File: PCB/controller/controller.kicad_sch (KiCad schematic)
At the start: 14 parts, among them U1 Raspberry_Pi_Pico, X1 Switch, Y1 Switch

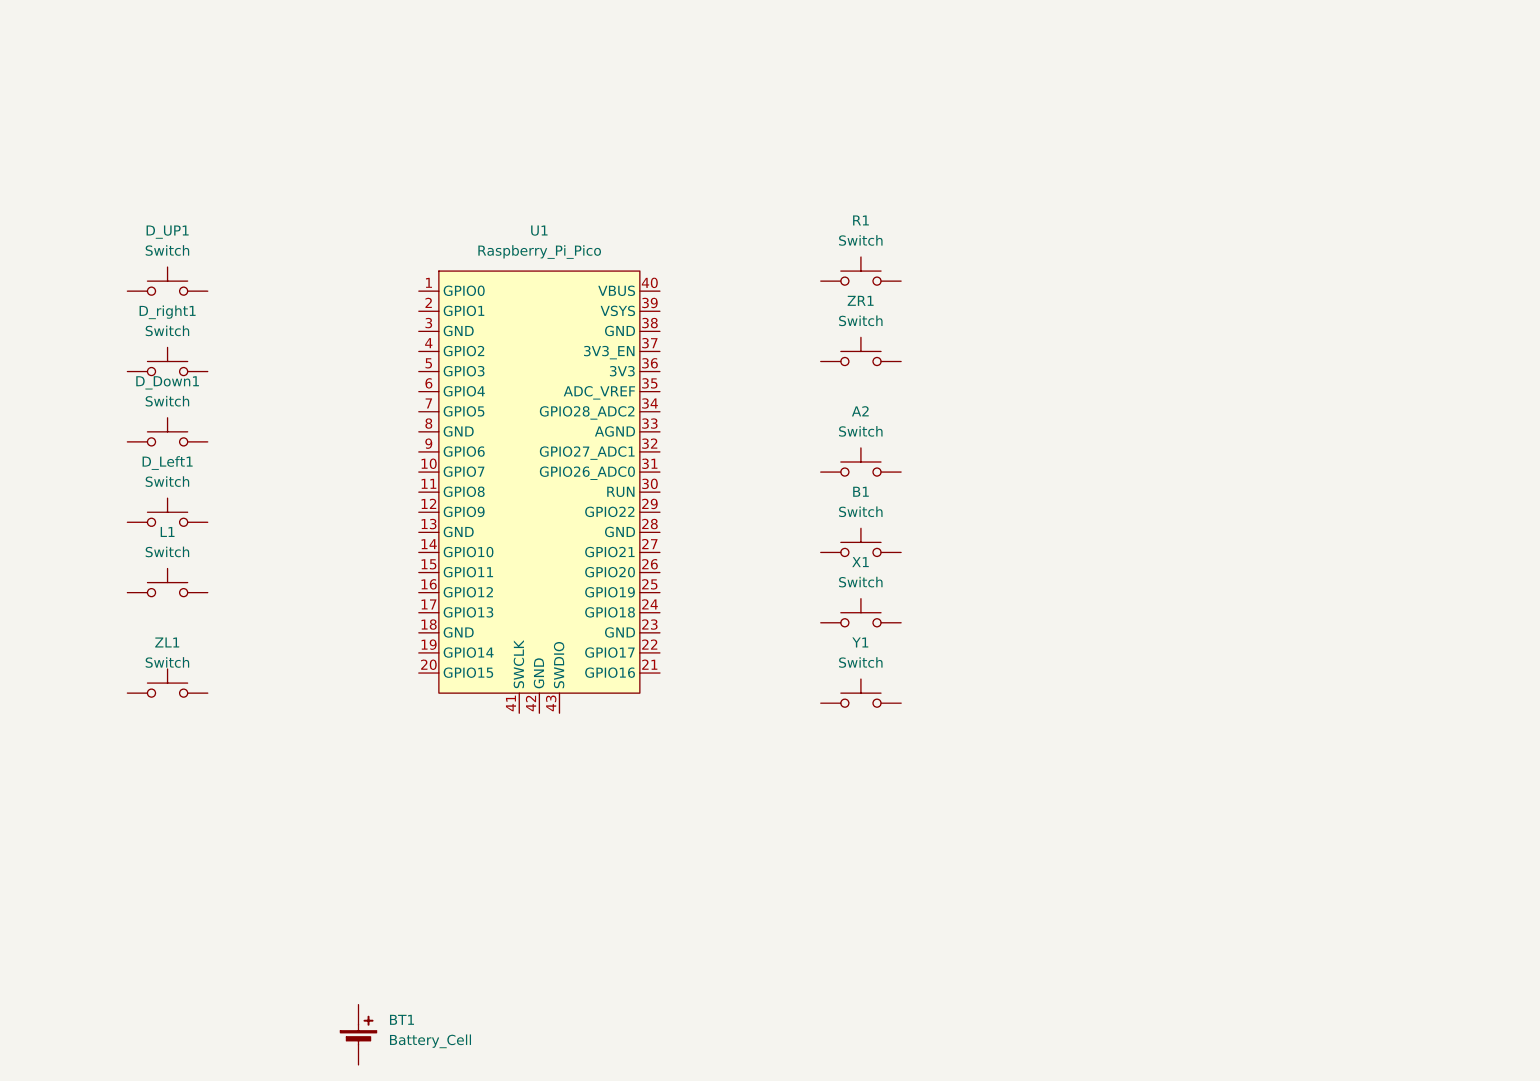
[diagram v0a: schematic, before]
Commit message: doin stuffs
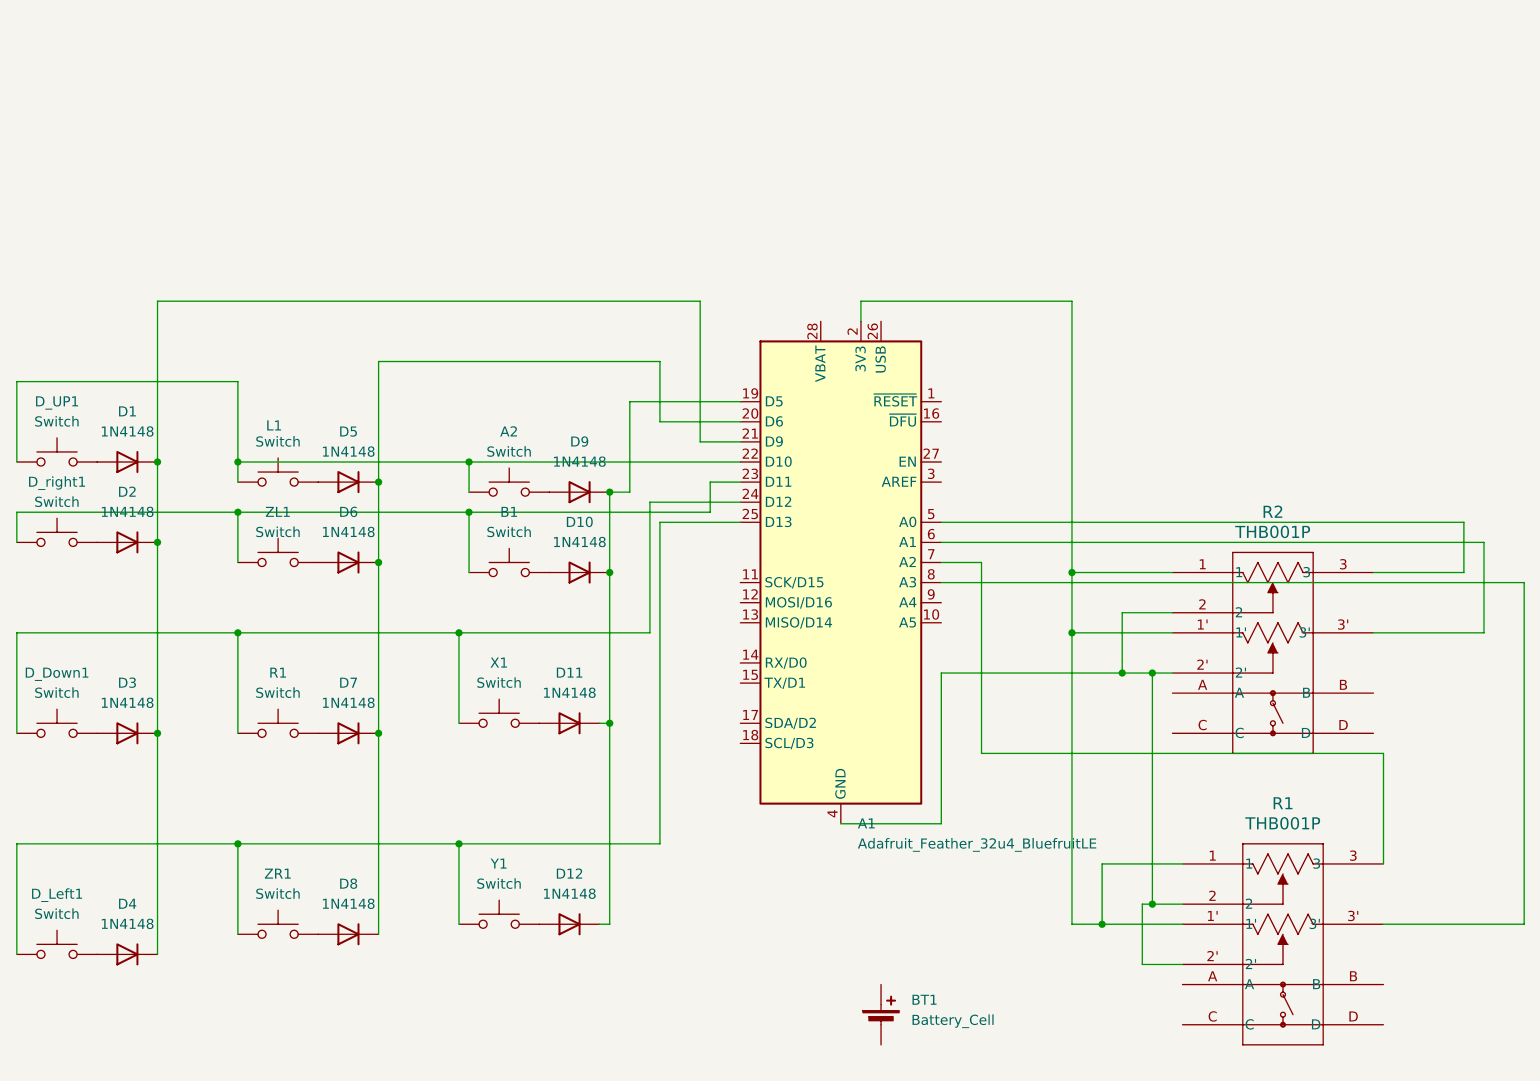
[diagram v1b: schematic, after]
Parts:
- removed U1: Raspberry_Pi_Pico, ScottoKeebs_MCU:Raspberry_Pi_Pico, symbol ScottoKeebs:MCU_Raspberry_Pi_Pico
- added A1: Adafruit_Feather_32u4_BluefruitLE, Module:Adafruit_Feather, symbol MCU_Module:Adafruit_Feather_32u4_BluefruitLE
- added D1, D10, D11, D12, D2, D3, D4, D5, D6, D7, D8, D9: 1N4148, Diode_THT:D_DO-35_SOD27_P7.62mm_Horizontal, symbol Diode:1N4148
- added R1, R2: THB001P, ScottoKeebs_Miscellaneous:THB001P_CNK, symbol 2025-05-29_23-49-57:THB001P
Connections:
- net at B1.1: now also D_right1.1, ZL1.1, A1.23 (D11)
- net at B1.2: now also D10.2 (A)
- net at A2.1: now also D_UP1.1, L1.1, A1.22 (D10)
- net at A2.2: now also D9.2 (A)
- net at ZR1.1: now also D_Left1.1, Y1.1, A1.25 (D13)
- net at ZR1.2: now also D8.2 (A)
- net at R1.1: now also D_Down1.1, X1.1, A1.24 (D12)
- net at R1.2: now also D7.2 (A)
- net at Y1.2: now also D12.2 (A)
- net at D_Down1.2: now also D3.2 (A)
- net at ZL1.2: now also D6.2 (A)
- net at D_right1.2: now also D2.2 (A)
- net at D_Left1.2: now also D4.2 (A)
- net at D_UP1.2: now also D1.2 (A)
- net at X1.2: now also D11.2 (A)
- net at L1.2: now also D5.2 (A)
- new net: A1.19 (D5), D10.1 (K), D11.1 (K), D12.1 (K), D9.1 (K)
- new net: A1.2 (3V3), R1.1, R1.1', R2.1, R2.1'
- new net: A1.20 (D6), D5.1 (K), D6.1 (K), D7.1 (K), D8.1 (K)
- new net: A1.21 (D9), D1.1 (K), D2.1 (K), D3.1 (K), D4.1 (K)
- new net: A1.4 (GND), R1.2, R1.2', R2.2, R2.2'
- new net: A1.5 (A0), R2.3
- new net: A1.6 (A1), R2.3'
- new net: A1.7 (A2), R1.3
- new net: A1.8 (A3), R1.3'
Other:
- moved on the sheet: A2, B1, BT1, D_Down1, D_Left1, D_UP1, D_right1, L1, R1, X1, Y1, ZL1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

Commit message: more work
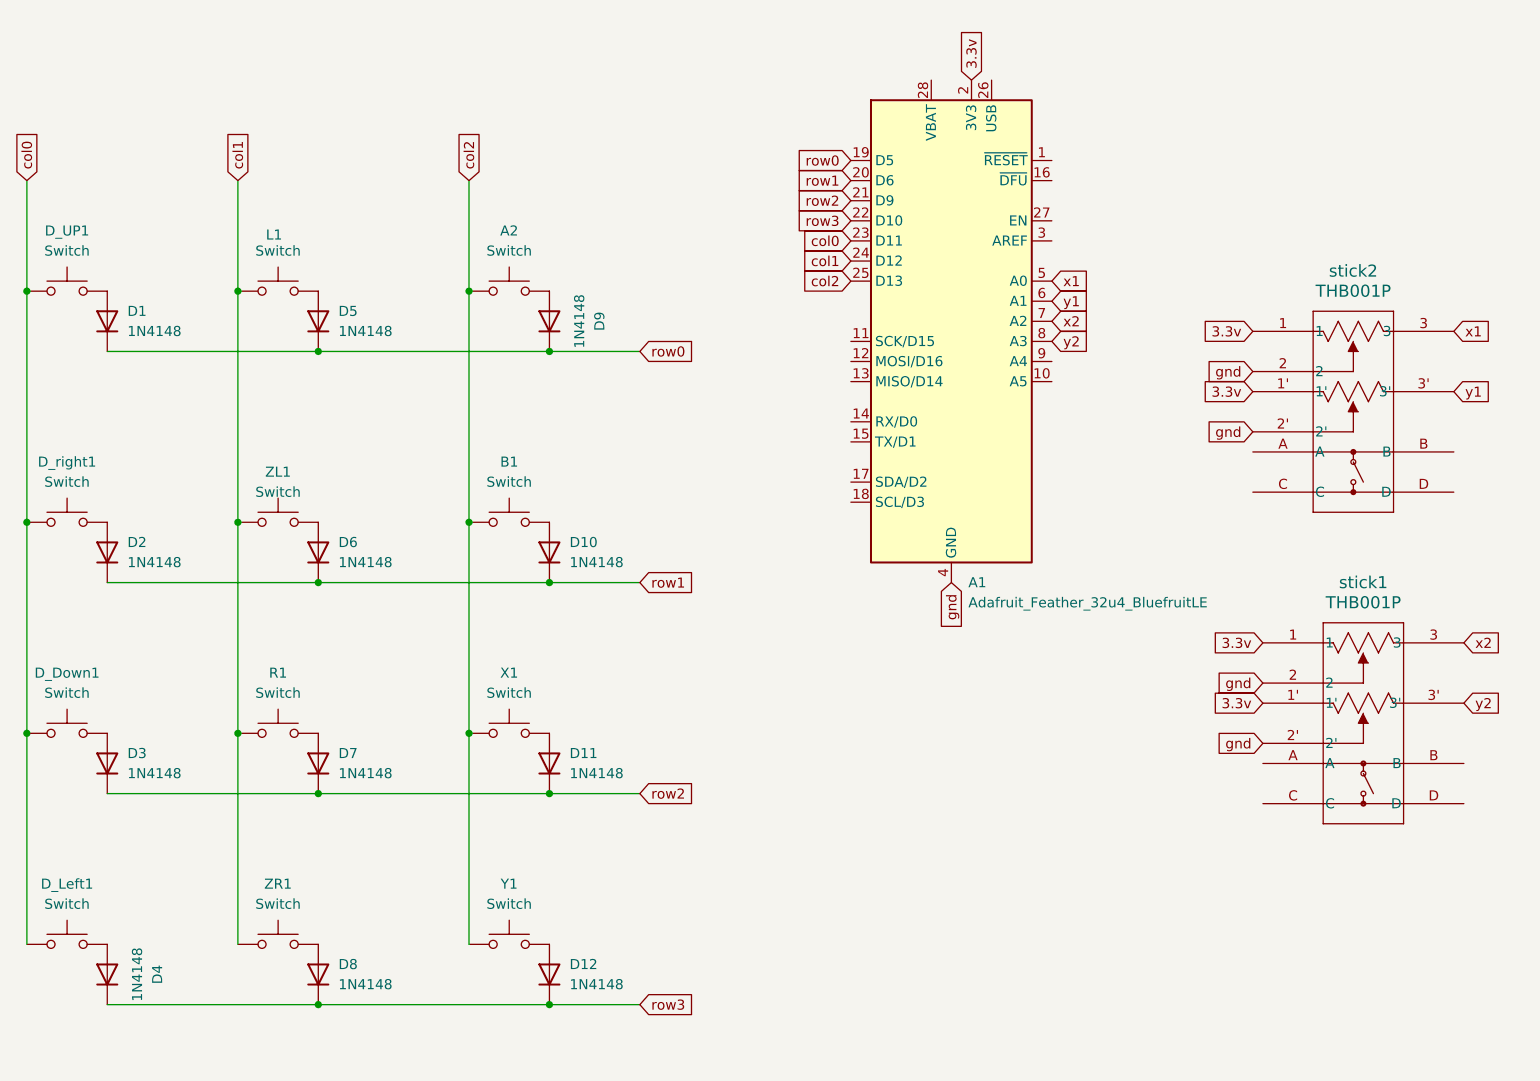
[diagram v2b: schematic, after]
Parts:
- removed BT1: Battery_Cell, Battery:BatteryHolder_Bulgin_BX0034_1xAAA, symbol Device:Battery_Cell
- renumbered R1 to stick1, R2 to stick2
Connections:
- net col0: now reaches A1.23 (D11), D_right1.1
- net col0: now also D_Down1.1, D_Left1.1, D_UP1.1; no longer B1.1, ZL1.1
- net 3.3v: now reaches A1.2 (3V3), stick1.1, stick1.1', stick2.1, stick2.1'
- net col1: now reaches A1.24 (D12), R1.1
- net col1: now also L1.1, ZL1.1, ZR1.1; no longer D_Down1.1, X1.1
- net col2: now reaches A1.25 (D13), Y1.1
- net col2: now also A2.1, B1.1, X1.1; no longer D_Left1.1, ZR1.1
- net gnd: now reaches A1.4 (GND), stick1.2, stick1.2', stick2.2, stick2.2'
- net x1: now reaches A1.5 (A0), stick2.3
- net y1: now reaches A1.6 (A1), stick2.3'
- net x2: now reaches A1.7 (A2), stick1.3
- net y2: now reaches A1.8 (A3), stick1.3'
- new net row0: A1.19 (D5), D1.1 (K), D5.1 (K), D9.1 (K)
- new net row1: A1.20 (D6), D10.1 (K), D2.1 (K), D6.1 (K)
- new net row2: A1.21 (D9), D11.1 (K), D3.1 (K), D7.1 (K)
- new net row3: A1.22 (D10), D12.1 (K), D4.1 (K), D8.1 (K)
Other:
- moved on the sheet: A1, A2, B1, D1, D10, D11, D12, D2, D3, D4, D5, D6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
